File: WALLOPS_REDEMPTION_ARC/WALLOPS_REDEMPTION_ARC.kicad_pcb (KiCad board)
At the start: 2 copper layers, 57.1 x 72.6 mm, 103 parts, among them J1 Power Connector, J2 I2C Connector, U1 TCA9517DR, U10 ISM330DHCX, U2 AP2112K-1.8, U3 5V to 3.3V Converter, U4 VL53L8CXV0GC/1, U5 Schottky Diode, U6 SN74LVC125ADR, U7 VL53L8CXV0GC/1, U8 VL53L8CXV0GC/1, U9 VL53L8CXV0GC/1

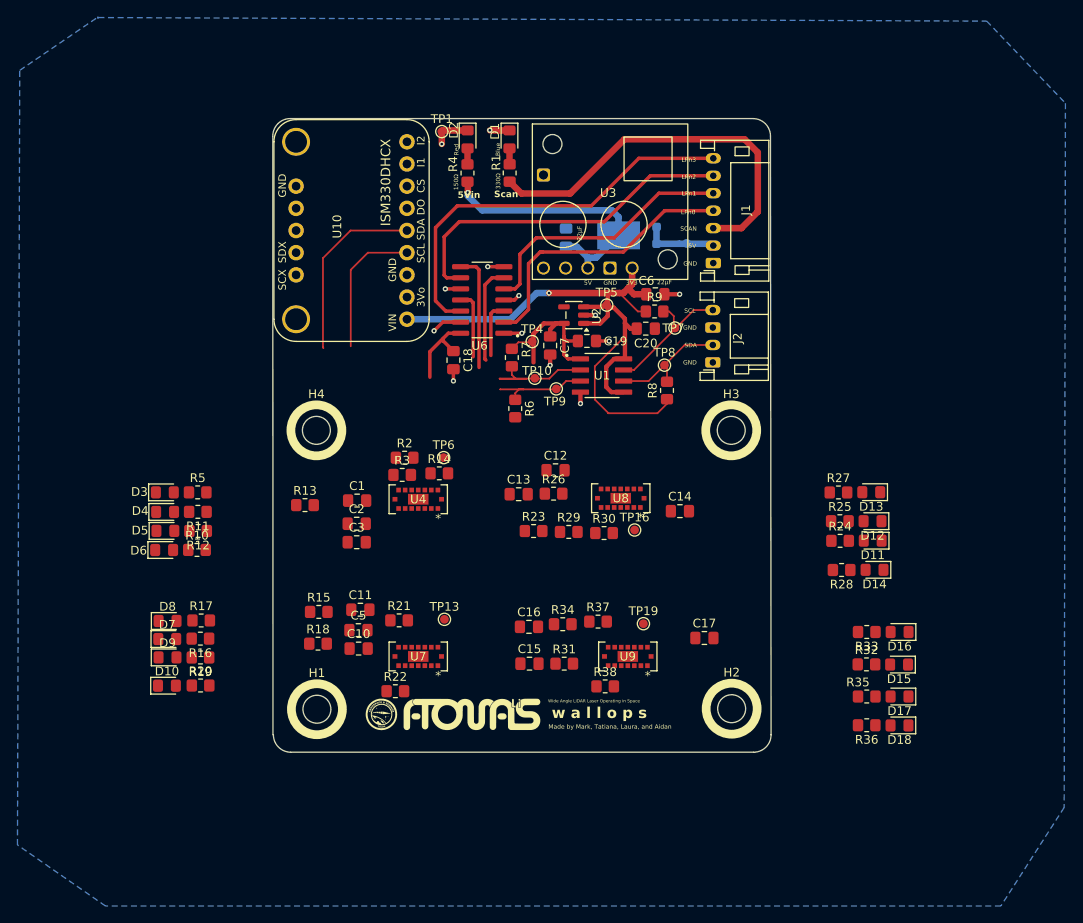
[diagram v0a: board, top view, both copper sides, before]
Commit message: Updated Wallops Redemption ARC
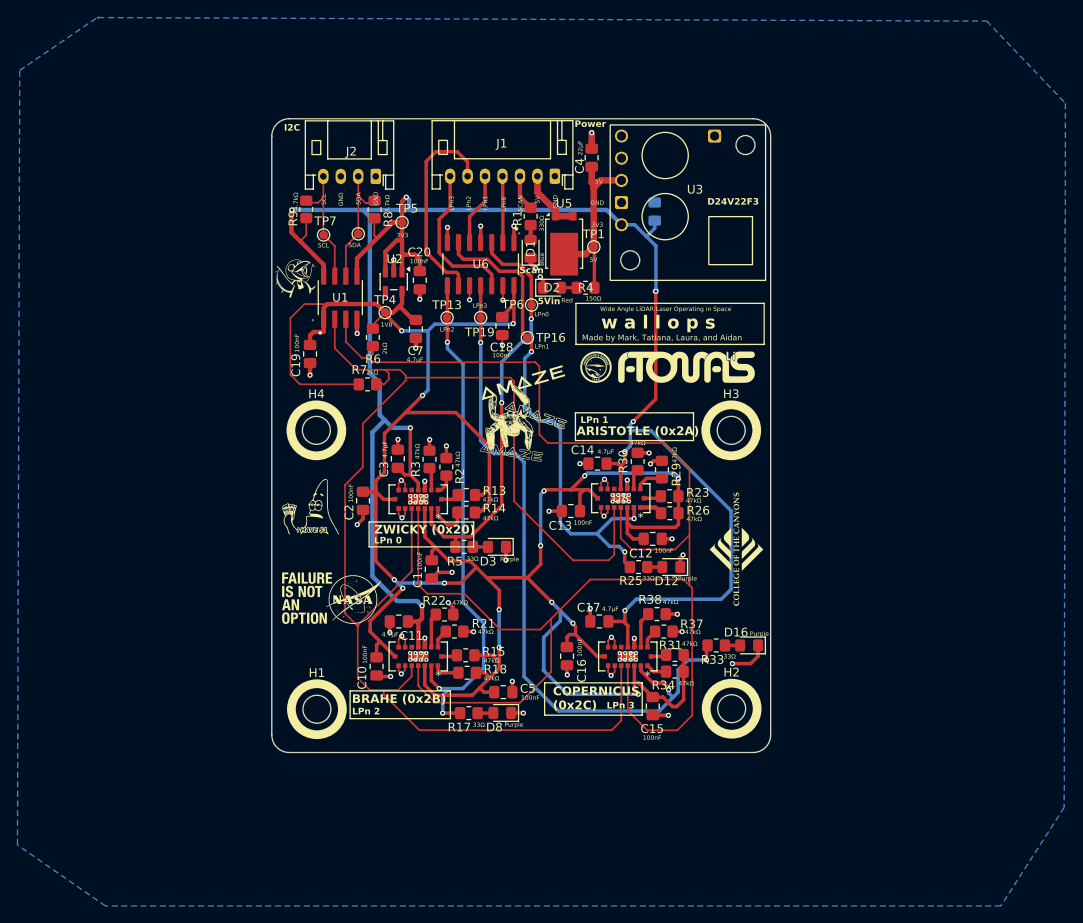
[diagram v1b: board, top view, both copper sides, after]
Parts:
- removed D10, D14, D18, D6: GREEN_LED, LED_SMD:LED_0805_2012Metric_Pad1.15x1.40mm_HandSolder
- removed D11, D13, D15, D17, D4, D5, D7, D9: RED_LED, LED_SMD:LED_0805_2012Metric_Pad1.15x1.40mm_HandSolder
- removed R10, R20, R28, R36: 120 Ω, Resistor_SMD:R_0805_2012Metric_Pad1.20x1.40mm_HandSolder
- removed R11, R12, R16, R19, R24, R27, R32, R35: 22Ω, Resistor_SMD:R_0805_2012Metric_Pad1.20x1.40mm_HandSolder
- removed TP10: 1SC_TP, TestPoint:TestPoint_Pad_D1.0mm
- removed TP2: 5V_TP, TestPoint:TestPoint_Pad_D1.0mm
- removed TP9: 1SD_TP, TestPoint:TestPoint_Pad_D1.0mm
- removed U10: ISM330DHCX, RockSat:ISM330DHCX
- added G***: LOGO, LOGO, F.Cu at (142.4, 110.7)
- added G***: LOGO, LOGO, F.Cu at (118.0, 95.2)
- added G***: LOGO, LOGO, F.Cu at (92.0, 79.5)
- added G***: LOGO, LOGO, F.Cu at (96.0, 116.3)
- added G***: LOGO, LOGO, F.Cu at (93.7, 105.8)
- added G***: LOGO, LOGO, B.Cu at (119.2, 86.5)
- C4, U5: moved to F.Cu
- C6: moved to B.Cu
- TP1: value GND_TP -> 5V_TP
- TP8: value SD_TP -> SDA_TP
- moved G*** 46.7 mm to (134.6, 89.9)
- moved J2 44.1 mm to (101.1, 68.0), turned to 180 degrees
- moved TP7 41.6 mm to (95.2, 74.7)
- moved R9 41.6 mm to (93.2, 71.8), turned to 90 degrees
- moved D8 39.8 mm to (115.6, 129.5), turned to 180 degrees
- moved TP19 39.7 mm to (113.2, 84.2)
- moved R8 39.4 mm to (101.0, 71.8)
- moved D3 38.5 mm to (115.0, 110.5), turned to 180 degrees
- moved TP8 38.2 mm to (99.1, 74.6)
- moved TP13 34.6 mm to (109.3, 84.2)
- moved R17 32.4 mm to (111.8, 129.5), turned to 180 degrees
- moved C19 31.7 mm to (93.6, 88.4), turned to 90 degrees
- moved U1 31.3 mm to (97.1, 81.9), turned to 90 degrees
- moved R5 31.1 mm to (111.3, 110.5), turned to 180 degrees
- moved C20 26.5 mm to (106.2, 79.9), turned to 90 degrees
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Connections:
- J1 pad 2: /5V -> /5Vin
- J1 pad 4: /LPn_0 -> /LPn_0_3V3
- J1 pad 5: /LPn_1 -> /LPn_1_3V3
- J1 pad 6: /LPn_2 -> /LPn_2_3V3
- J1 pad 7: /LPn_3 -> /LPn_3_3V3
- J2 pad 2: /SDA -> /SDA_3V3
- J2 pad 4: /SCL -> /SCL_3V3
- R8 pad 2: /SDA -> /SDA_3V3
- R9 pad 2: /SCL -> /SCL_3V3
- TP1 pad 1: GND -> /5V
- TP7 pad 1: /SCL -> /SCL_3V3
- TP8 pad 1: /SDA -> /SDA_3V3
- U1 pad 6: /SDA -> /SDA_3V3
- U1 pad 7: /SCL -> /SCL_3V3
- U5 pad 1: /5V -> /5Vin
- U5 pad 2: /5V -> /5Vin
- U6 pad 12: /LPn_3 -> /LPn_3_3V3
- U6 pad 2: /LPn_0 -> /LPn_0_3V3
- U6 pad 5: /LPn_1 -> /LPn_1_3V3
- U6 pad 9: /LPn_2 -> /LPn_2_3V3
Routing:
- net /1V8: track 29.6 -> 296.5 mm, vias 0 -> 15
- net /3V3: track 78.6 -> 232.4 mm, vias 1 -> 8
- net /SDA: track 46.7 -> 179.6 mm
- net /SCL: track 46.5 -> 160.9 mm
- net GND: track 26.4 -> 83.9 mm, vias 13 -> 82
- net /SCAN: track 44.8 -> 4.11 mm
- net /LPn_3: track 54.6 -> 84.3 mm, vias 0 -> 3
- net /LPn_2_3V3: track 0.00 -> 24.1 mm
- net /5V: track 39.2 -> 21.1 mm, vias 1 -> 0
- net /LPn_3_3V3: track 0.00 -> 17.3 mm
- net /LPn_1: track 41.7 -> 58.3 mm, vias 0 -> 3
- net /SDA_3V3: track 0.00 -> 14.2 mm
- net /SCL_3V3: track 0.00 -> 14.1 mm
- net /LPn_0: track 38.7 -> 48.0 mm, vias 0 -> 2
- net /LPn_1_3V3: track 0.00 -> 8.04 mm
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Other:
- outline, holes or cut-outs redrawn
- board text added: "*"
- board text added: "100nF"
- board text added: "1V8"
- board text added: "2kΩ"
- board text added: "33Ω"
- board text added: "4.7kΩ"
- board text added: "4.7μF"
- board text added: "47kΩ"
- board text added: "ARISTOTLE (0x2A)"
- board text added: "BRAHE (0x2B)"
- board text added: "COPERNICUS (0x2C)"
- board text added: "D24V22F3"
- board text added: "I2C"
- board text added: "LPn 0"
- board text added: "LPn 1"
- board text added: "LPn 2"
- board text added: "LPn 3"
- board text added: "Power"
- board text added: "Purple"
- board text added: "ZWICKY (0x20)"
